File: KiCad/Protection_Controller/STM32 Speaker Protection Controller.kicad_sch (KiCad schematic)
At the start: 58 parts, among them J1 AC1, J10 SPEAKER_OUT_R, J3 AC2, J5 AMP_OUT_L, J6 AMP_OUT_R, J8 SPEAKER_OUT_L, K1 G2RL-1A-E DC12, K2 G2RL-1A-E DC12, Q1 BC337, Q2 BC337, SW1 MUTE / ENABLE, SW2 FAULT RESET, T1 FS24-1500-C2, U1 LM7812, U2 NUCLEO-G031K8

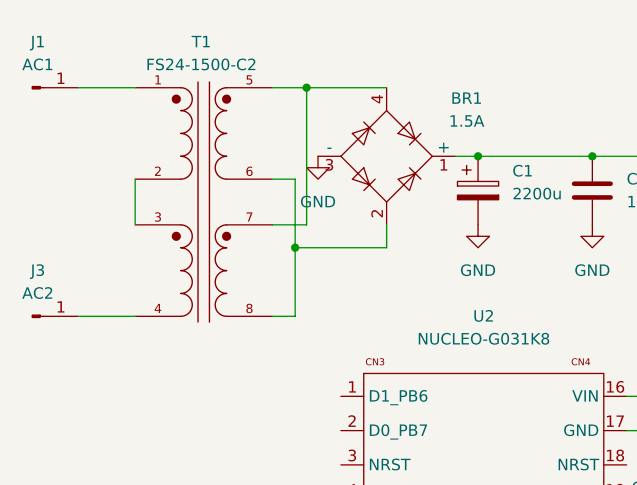
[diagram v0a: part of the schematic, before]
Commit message: Add files via upload
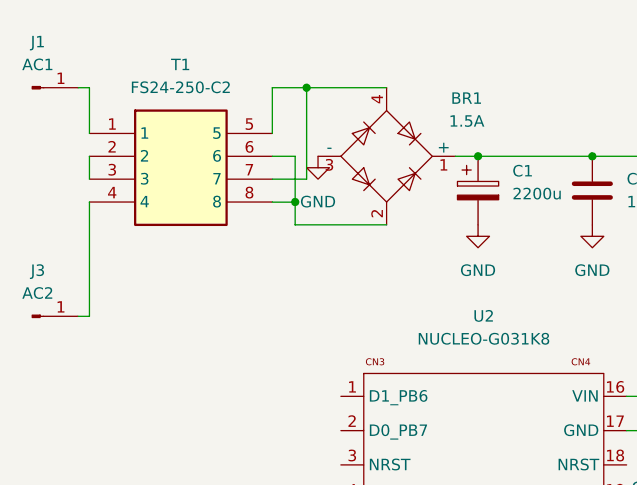
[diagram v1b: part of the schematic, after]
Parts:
- removed T1: FS24-1500-C2, FS24-1500-C2:TRANSFORMER_FS24-1500-C2, symbol FS24-1500-C2:FS24-1500-C2
- added T1: FS24-250-C2, FS24250C2, symbol FS24-250-C2:FS24-250-C2
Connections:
- net at J1.1 (Pin_1): now also T1.1
- net at BR1.2: now also T1.6, T1.8
- net at BR1.4: now also T1.5, T1.7
- net at J3.1 (Pin_1): now also T1.4
- new net: T1.2, T1.3
